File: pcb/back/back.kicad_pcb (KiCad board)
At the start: 4 copper layers, 26.5 x 26.5 mm, 60 parts, among them J1 Conn_01x02, J2 USB_B_Micro, U1 ATSAMD21G18A-A, U2 LSM6DS3, U3 XC6206PxxxMR, U4 TP4057

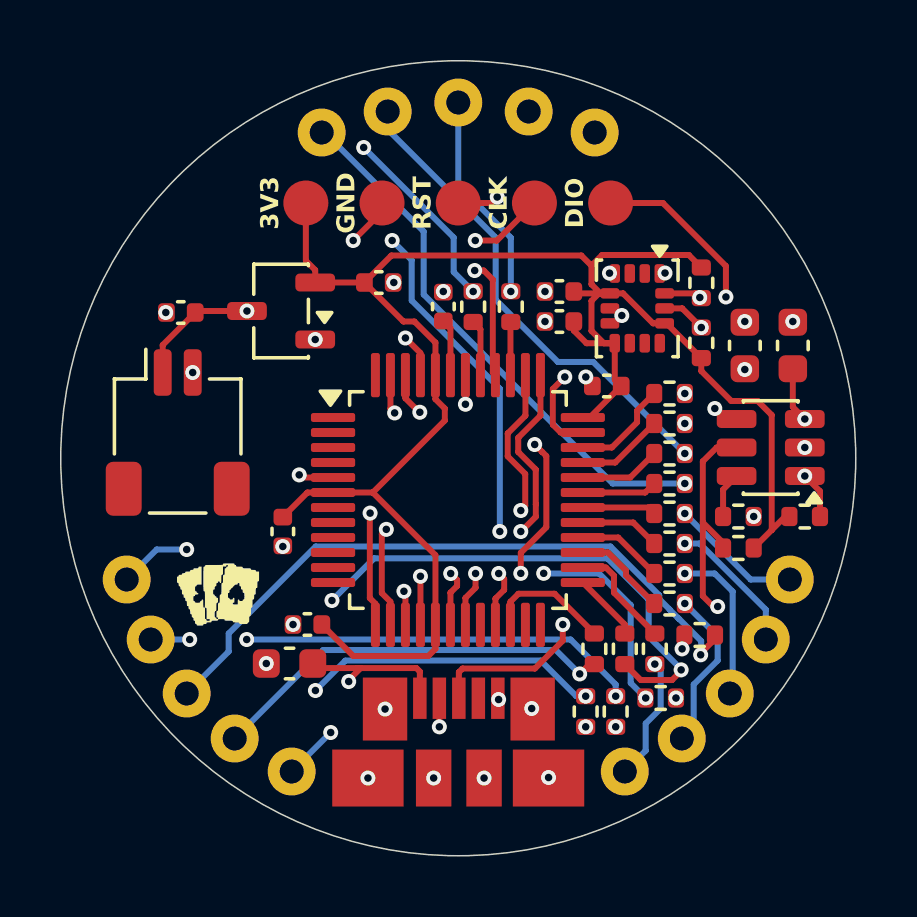
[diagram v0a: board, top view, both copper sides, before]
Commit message: Update accelerometer
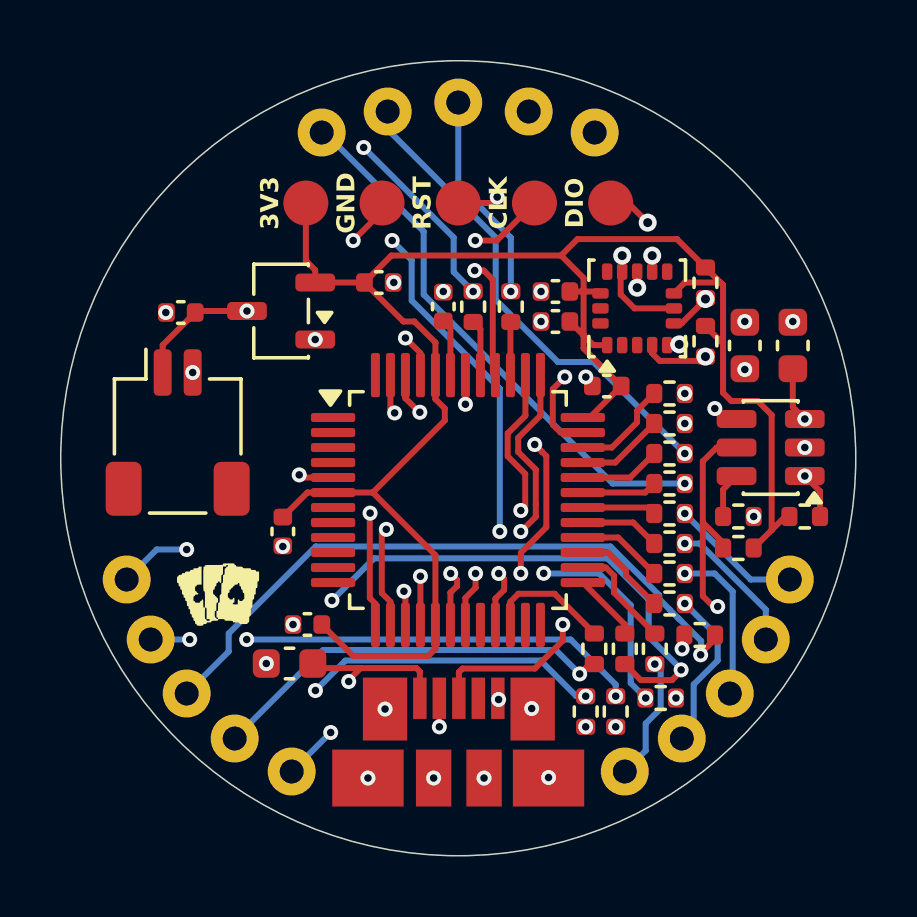
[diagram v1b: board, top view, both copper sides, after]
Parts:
- U2: value LSM6DS3 -> LIS3DH; footprint Package_LGA:LGA-14_3x2.5mm_P0.5mm_LayoutBorder3x4y -> Package_LGA:LGA-16_3x3mm_P0.5mm_LayoutBorder3x5y
- moved R19 0.15 mm to (159.0, 91.5), turned to -90 degrees
- moved R18 0.14 mm to (159.0, 89.6)
- moved C5 0.13 mm to (154.0, 89.9)
- moved C6 0.13 mm to (154.0, 90.9)
- turned U2 to 90 degrees
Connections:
- U2 pad 1: GND -> +3V3
- U2 pad 10: unconnected-(U2-NC-Pad10) -> GND
- U2 pad 11: unconnected-(U2-NC-Pad11) -> /AINT
- U2 pad 12: +3V3 -> GND
- U2 pad 13: /SCL -> unconnected-(U2-ADC3-Pad13)
- U2 pad 14: /SDA -> +3V3
- U2 pad 4: /AINT -> /SCL
- U2 pad 5: +3V3 -> GND
- U2 pad 6: GND -> /SDA
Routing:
- net /SWDIO: track 19.5 -> 16.0 mm
- net GND: track 10.4 -> 13.4 mm, vias 29 -> 30
- net +3V3: track 62.5 -> 63.9 mm
- net /AINT: track 11.1 -> 11.7 mm
